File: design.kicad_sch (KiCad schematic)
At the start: 4 parts, among them J1 490107670412, U1 CH340C, U2 TS3USB30RSWR, U3 CH340C

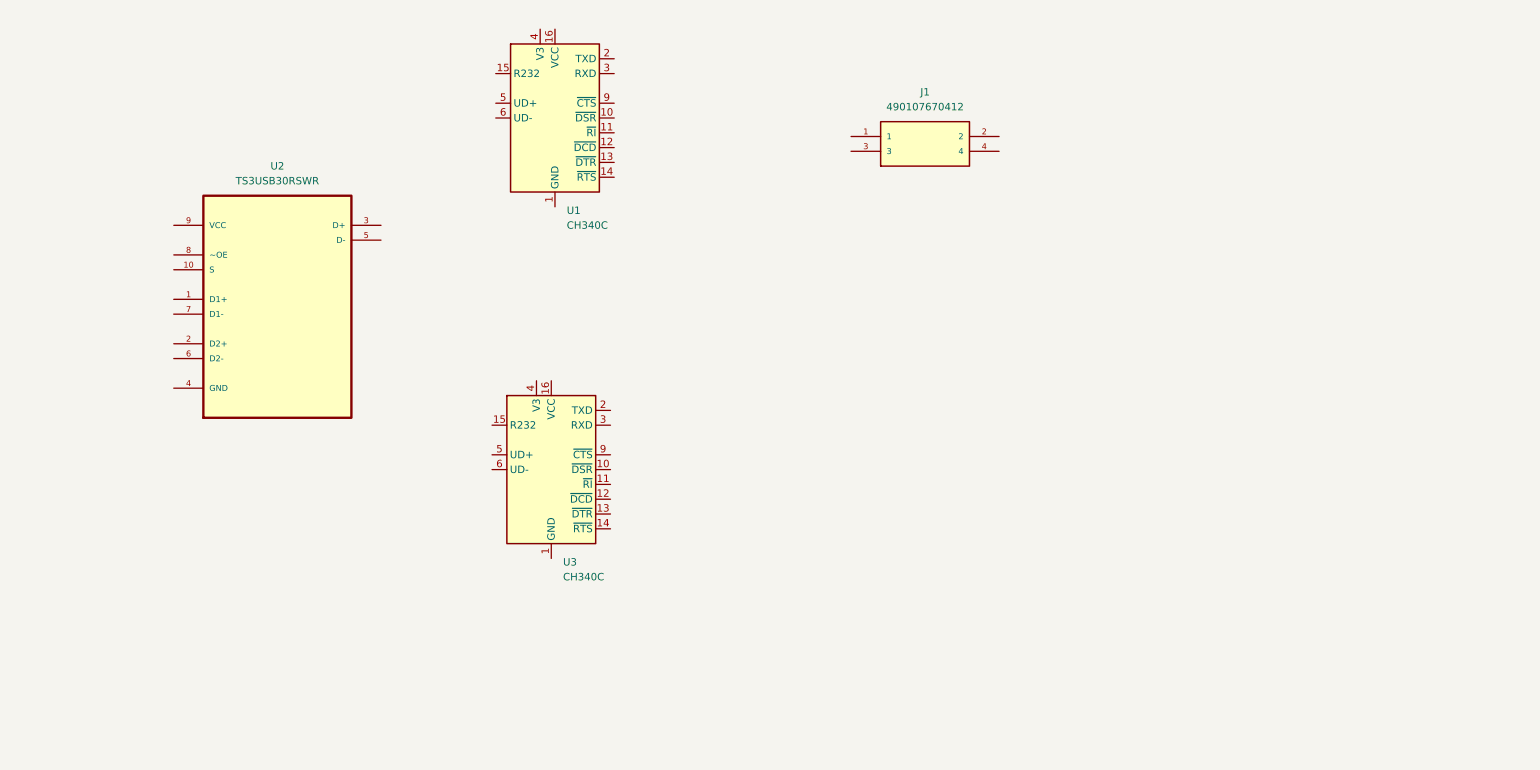
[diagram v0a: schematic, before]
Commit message: add components
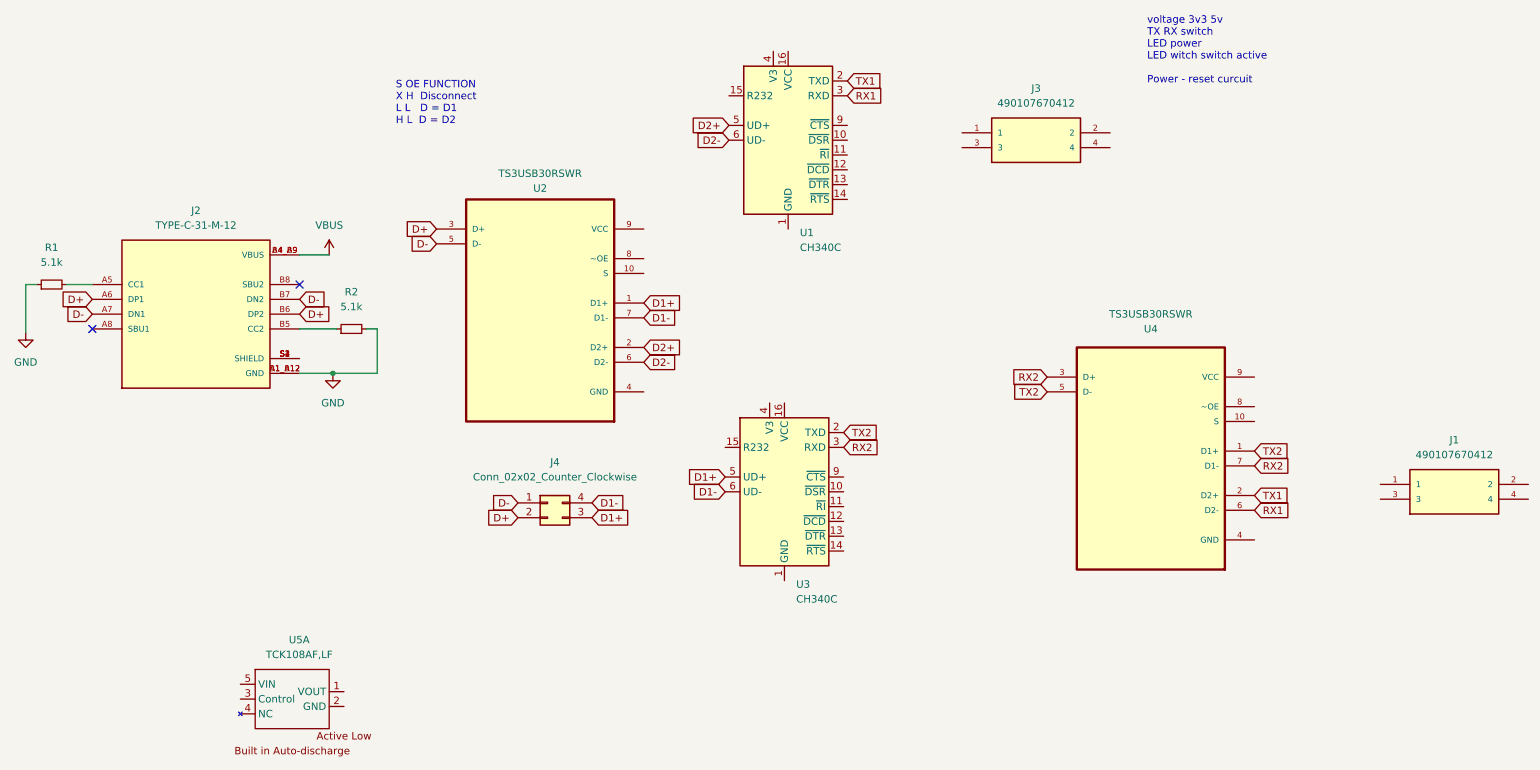
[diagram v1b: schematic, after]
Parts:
- added J2: TYPE-C-31-M-12, Snapeda:TYPE-C-31-M-12_HRO_TYPE-C-31-M-12, symbol Snapeda:TYPE-C-31-M-12
- added J3: 490107670412, Snapeda:490107670412_WURTH_490107670412, symbol Snapeda:490107670412
- added J4: Conn_02x02_Counter_Clockwise, Connector_PinHeader_2.54mm:PinHeader_2x02_P2.54mm_Vertical, symbol Connector_Generic:Conn_02x02_Counter_Clockwise
- added R1, R2: 5.1k, Resistor_SMD:R_0805_2012Metric, symbol Device:R_Small
- added U4: TS3USB30RSWR, Snapeda:TS3USB30RSWR_QFN40P140X180X55-10N, symbol Snapeda:TS3USB30RSWR
- added U5: TCK108AF,LF, Package_TO_SOT_SMD:SOT-23-5, symbol Power_Management_custom:TCK108AF,LF
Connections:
- net D1+: now reaches U2.1 (D1+)
- net D1+: now also U3.5 (UD+), J4.3 (Pin_3)
- net D2+: now reaches U2.2 (D2+)
- net D2+: now also U1.5 (UD+)
- net D+: now reaches U2.3 (D+)
- net D+: now also J2.A6 (DP1), J2.B6 (DP2), J4.2 (Pin_2)
- net D-: now reaches U2.5 (D-)
- net D-: now also J2.A7 (DN1), J2.B7 (DN2), J4.1 (Pin_1)
- net D2-: now reaches U2.6 (D2-)
- net D2-: now also U1.6 (UD-)
- net D1-: now reaches U2.7 (D1-)
- net D1-: now also U3.6 (UD-), J4.4 (Pin_4)
- net TX2: now reaches U3.2 (TXD)
- net TX2: now also U4.1 (D1+), U4.5 (D-)
- net RX2: now reaches U3.3 (RXD)
- net RX2: now also U4.3 (D+), U4.7 (D1-)
- net TX1: now reaches U1.2 (TXD)
- net TX1: now also U4.2 (D2+)
- net RX1: now reaches U1.3 (RXD)
- net RX1: now also U4.6 (D2-)
- new net: J2.A5 (CC1), R1.2
- new net: J2.B5 (CC2), R2.1
- new net: J2.S1 (SHIELD), J2.S2 (SHIELD), J2.S3 (SHIELD), J2.S4 (SHIELD)
- new net GND: J2.A1_B12 (GND), J2.B1_A12 (GND), R1.1, R2.2
- new net VBUS: J2.A4_B9 (VBUS), J2.B4_A9 (VBUS)
- no-connect marks 0 -> 2
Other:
- note added: "S OE FUNCTION X H Disconnect L L D = D1 H L D = D2"
- note added: "voltage 3v3 5v TX RX switch LED power LED witch switch active Power - reset curcuit"
- moved on the sheet: J1, U1, U2, U3
